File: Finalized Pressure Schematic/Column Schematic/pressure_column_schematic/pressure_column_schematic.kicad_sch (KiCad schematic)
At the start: 0 parts

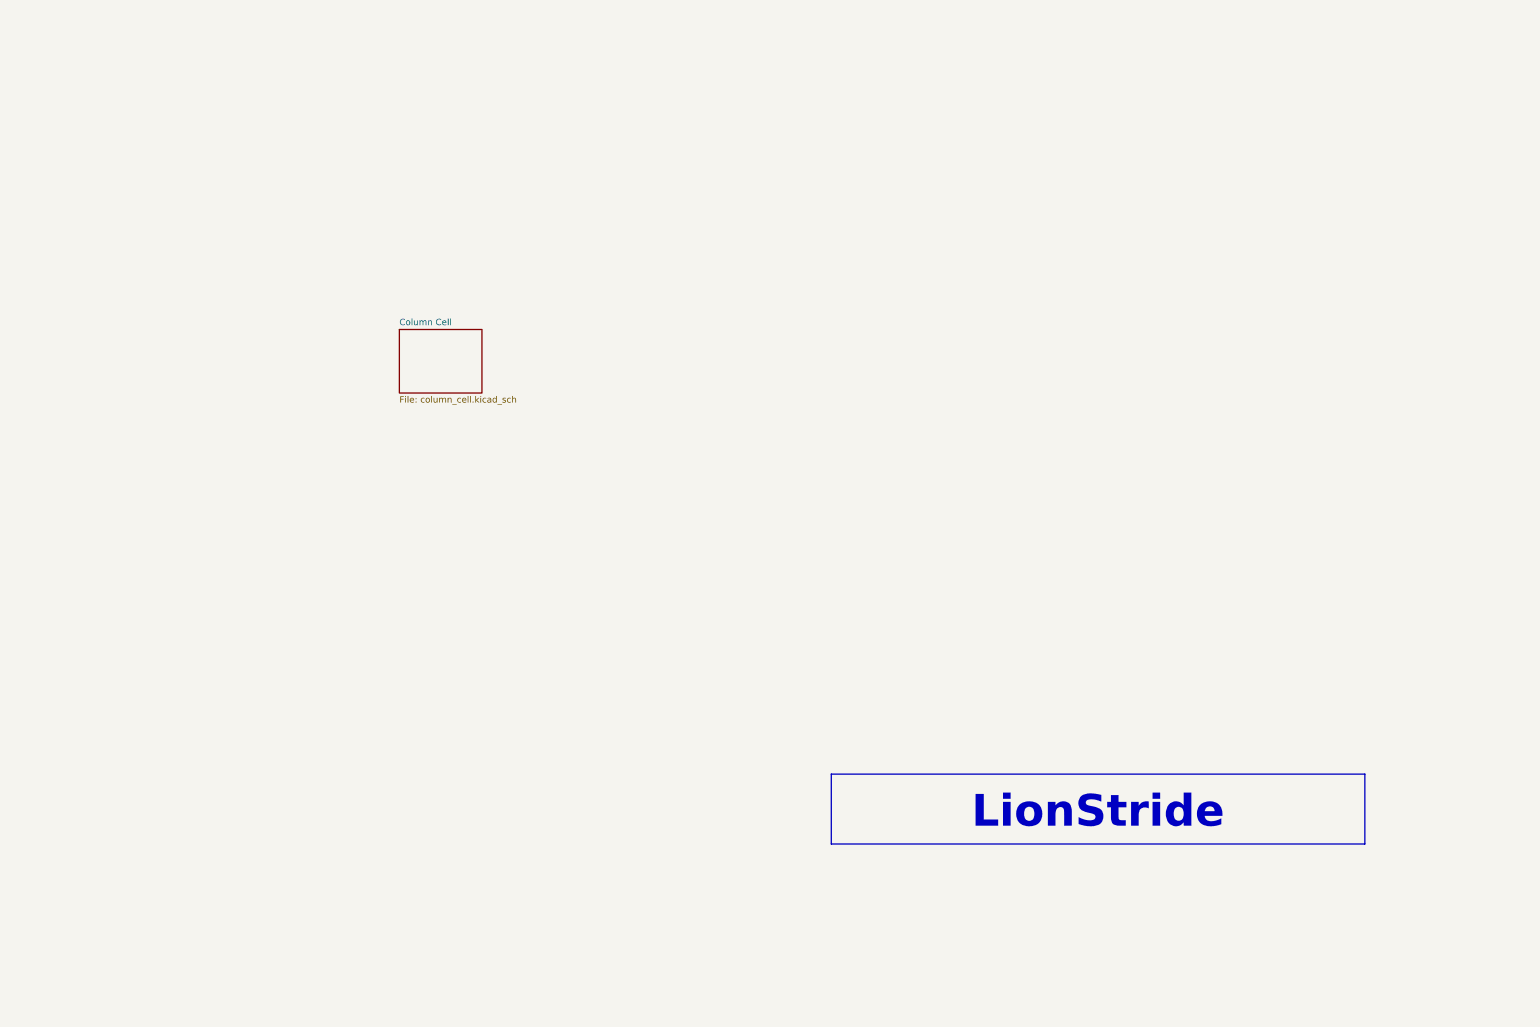
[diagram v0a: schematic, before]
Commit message: Work on V1
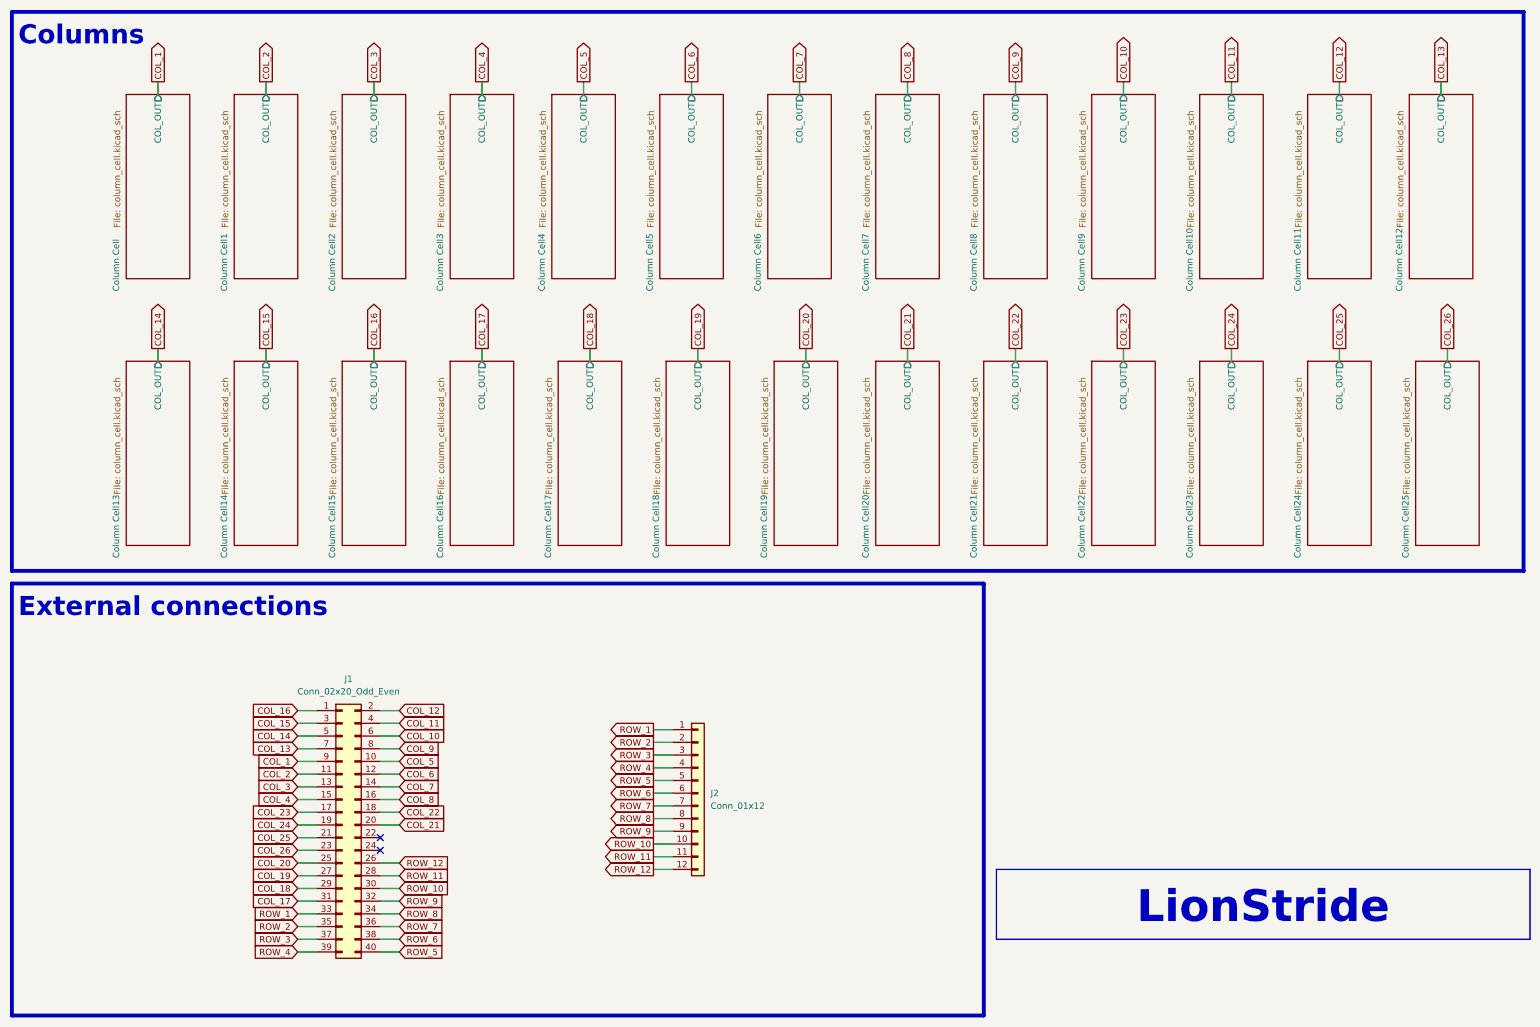
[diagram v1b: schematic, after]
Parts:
- added J1: Conn_02x20_Odd_Even, symbol Connector_Generic:Conn_02x20_Odd_Even
- added J2: Conn_01x12, symbol Connector_Generic:Conn_01x12
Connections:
- new net COL_1: J1.9 (Pin_9)
- new net COL_10: J1.6 (Pin_6)
- new net COL_11: J1.4 (Pin_4)
- new net COL_12: J1.2 (Pin_2)
- new net COL_13: J1.7 (Pin_7)
- new net COL_14: J1.5 (Pin_5)
- new net COL_15: J1.3 (Pin_3)
- new net COL_16: J1.1 (Pin_1)
- new net COL_17: J1.31 (Pin_31)
- new net COL_18: J1.29 (Pin_29)
- new net COL_19: J1.27 (Pin_27)
- new net COL_2: J1.11 (Pin_11)
- new net COL_20: J1.25 (Pin_25)
- new net COL_21: J1.20 (Pin_20)
- new net COL_22: J1.18 (Pin_18)
- new net COL_23: J1.17 (Pin_17)
- new net COL_24: J1.19 (Pin_19)
- new net COL_25: J1.21 (Pin_21)
- new net COL_26: J1.23 (Pin_23)
- new net COL_3: J1.13 (Pin_13)
- new net COL_4: J1.15 (Pin_15)
- new net COL_5: J1.10 (Pin_10)
- new net COL_6: J1.12 (Pin_12)
- new net COL_7: J1.14 (Pin_14)
- new net COL_8: J1.16 (Pin_16)
- new net COL_9: J1.8 (Pin_8)
- new net ROW_1: J1.33 (Pin_33), J2.1 (Pin_1)
- new net ROW_10: J1.30 (Pin_30), J2.10 (Pin_10)
- new net ROW_11: J1.28 (Pin_28), J2.11 (Pin_11)
- new net ROW_12: J1.26 (Pin_26), J2.12 (Pin_12)
- new net ROW_2: J1.35 (Pin_35), J2.2 (Pin_2)
- new net ROW_3: J1.37 (Pin_37), J2.3 (Pin_3)
- new net ROW_4: J1.39 (Pin_39), J2.4 (Pin_4)
- new net ROW_5: J1.40 (Pin_40), J2.5 (Pin_5)
- new net ROW_6: J1.38 (Pin_38), J2.6 (Pin_6)
- new net ROW_7: J1.36 (Pin_36), J2.7 (Pin_7)
- new net ROW_8: J1.34 (Pin_34), J2.8 (Pin_8)
- new net ROW_9: J1.32 (Pin_32), J2.9 (Pin_9)
- no-connect marks 0 -> 2
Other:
- added sheet Column Cell1 (column_cell.kicad_sch)
- added sheet Column Cell10 (column_cell.kicad_sch)
- added sheet Column Cell11 (column_cell.kicad_sch)
- added sheet Column Cell12 (column_cell.kicad_sch)
- added sheet Column Cell13 (column_cell.kicad_sch)
- added sheet Column Cell14 (column_cell.kicad_sch)
- added sheet Column Cell15 (column_cell.kicad_sch)
- added sheet Column Cell16 (column_cell.kicad_sch)
- added sheet Column Cell17 (column_cell.kicad_sch)
- added sheet Column Cell18 (column_cell.kicad_sch)
- added sheet Column Cell19 (column_cell.kicad_sch)
- added sheet Column Cell2 (column_cell.kicad_sch)
- added sheet Column Cell20 (column_cell.kicad_sch)
- added sheet Column Cell21 (column_cell.kicad_sch)
- added sheet Column Cell22 (column_cell.kicad_sch)
- added sheet Column Cell23 (column_cell.kicad_sch)
- added sheet Column Cell24 (column_cell.kicad_sch)
- added sheet Column Cell25 (column_cell.kicad_sch)
- added sheet Column Cell3 (column_cell.kicad_sch)
- added sheet Column Cell4 (column_cell.kicad_sch)
- added sheet Column Cell5 (column_cell.kicad_sch)
- added sheet Column Cell6 (column_cell.kicad_sch)
- added sheet Column Cell7 (column_cell.kicad_sch)
- added sheet Column Cell8 (column_cell.kicad_sch)
- added sheet Column Cell9 (column_cell.kicad_sch)
- sheet Column Cell ports: added COL_OUT; removed none
- note added: "Columns"
- note added: "External connections"
- title: (none) -> Pressure Column Schematic
